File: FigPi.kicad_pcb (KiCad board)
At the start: 2 copper layers, 25.8 x 40.4 mm, 45 parts, among them J1 MOLEX_47346-100147346, J2 SPI0 / PWM2 / PWM3, J3 UART0 / PWM3 / PWM4, J4 STEMMA_1/QWIIC_1/I2C1/PMW1, J5 ADC / PWM5 / PWM6, J6 STEMMA_0/QWIIC_0/I2C0/PMW0, J7 PWR, SW1 KMS233GLFG, SW2 KMS233GLFG, U1 RP2040, U2 QSPI NOR FLASH 2MiB 2x3mm USO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, U3 AP2112K-3.3, U4 OT201612MJBA4SL

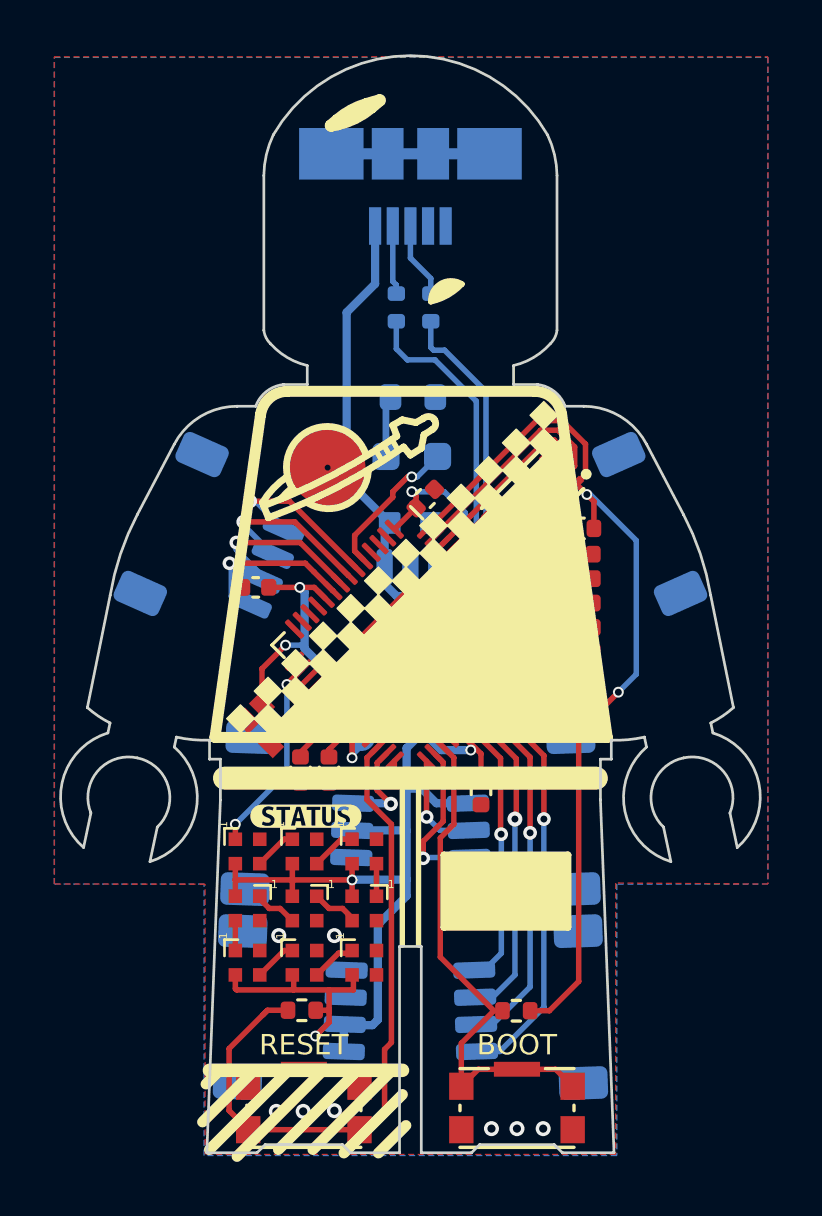
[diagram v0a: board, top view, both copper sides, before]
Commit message: Update to v2.3
Updated the schematic and board to v2.3.
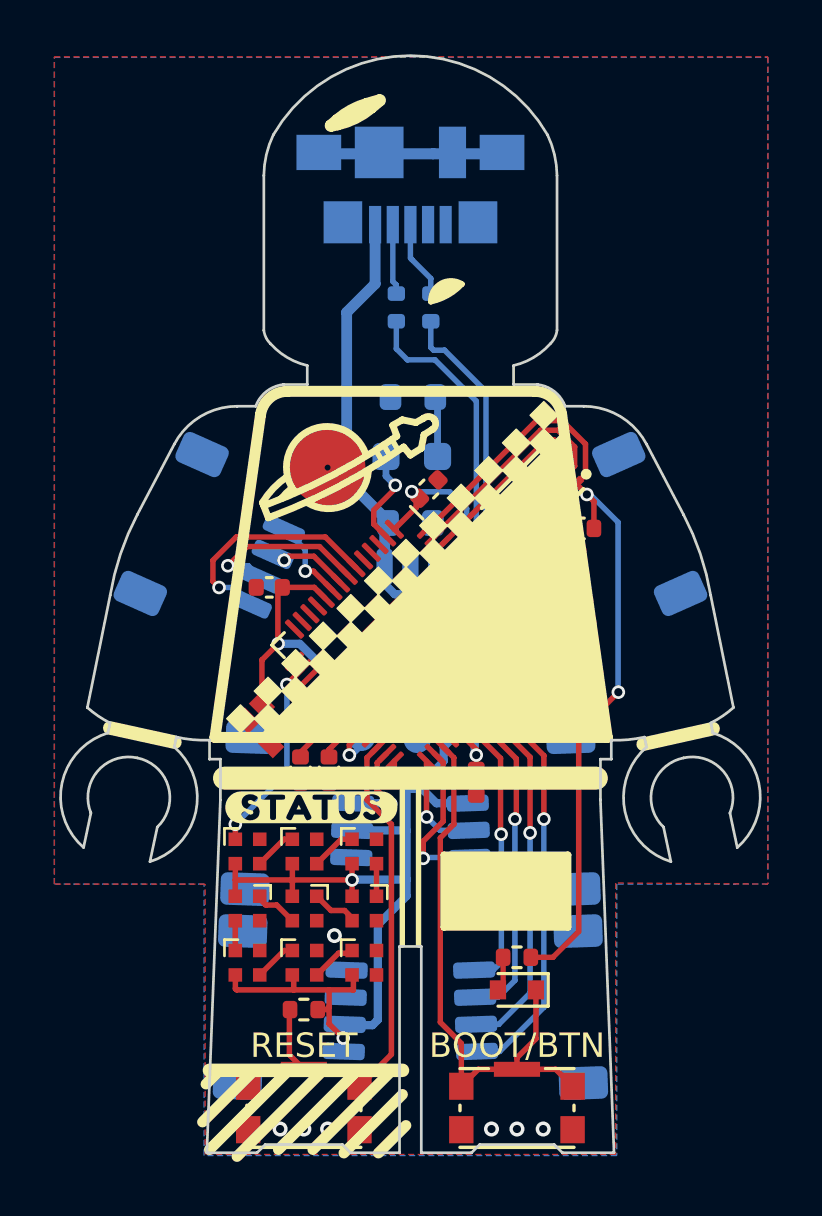
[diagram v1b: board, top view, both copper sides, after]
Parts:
- removed the J1 at (12.0, -36.8)
- removed kibuzzard-620D4CA4: G***, kibuzzard-620D4CA4
- added D11: RB520S-30, Diode_SMD:D_SOD-523, F.Cu at (15.9, -6.00)
- added J7: USB_B_Micro, Connector_USB:USB_Micro-B_Molex_47346-0001, B.Cu at (12.0, -35.6)
- added kibuzzard-640B746F: G***, kibuzzard-640B746F, F.Cu at (8.35, -12.7)
- added kibuzzard-640F7A39: G***, kibuzzard-640F7A39, B.Cu at (16.1, -16.5)
- added kibuzzard-640F7A5B: G***, kibuzzard-640F7A5B, B.Cu at (8.12, -16.5)
- added kibuzzard-640F7BF6: G***, kibuzzard-640F7BF6, B.Cu at (17.4, -26.2)
- added kibuzzard-640F7C1A: G***, kibuzzard-640F7C1A, B.Cu at (6.47, -26.4)
- added kibuzzard-640F7C6F: G***, kibuzzard-640F7C6F, B.Cu at (7.67, -1.18)
- added kibuzzard-640F7C7F: G***, kibuzzard-640F7C7F, B.Cu at (16.8, -1.15)
- added kibuzzard-640F7D7C: G***, kibuzzard-640F7D7C, B.Cu at (9.18, -32.5)
- C4: renamed from C9; footprint MINI_SAM_D51_r025_b001:0603_CAPACITOR -> Resistor_SMD:R_0603_1608Metric
- C5: renamed from C10; footprint MINI_SAM_D51_r025_b001:0603_CAPACITOR -> Resistor_SMD:R_0603_1608Metric
- SW1, SW2: value KMS233GLFG -> KMS231GLFG
- U2: value QSPI NOR FLASH 2MiB 2x3mm USON (W25Q16JVUXIQ) -> QSPI NOR FLASH 2MiB 2x3mm USON (W25Q16JVUXxQ)
- moved TP2 2.47 mm to (12.2, -15.2)
- moved R6 1.97 mm to (15.9, -7.20)
- moved C1 0.52 mm to (17.7, -22.1)
- moved C8 0.50 mm to (6.80, -20.8)
- moved C6 0.40 mm to (17.9, -21.1)
- moved C11 0.39 mm to (14.4, -13.7)
- moved C10 0.37 mm to (12.7, -24.4)
- moved C2 0.27 mm to (18.0, -20.2)
- moved C7 0.15 mm to (18.1, -19.4)
- moved C13 0.10 mm to (18.4, -17.6)
- moved R2 0.08 mm to (8.07, -5.28), turned to 0 degrees
- turned D10 to 180 degrees
- turned R1 to 180 degrees
- renumbered C11 to C10, C12 to C11, C13 to C12, C14 to C13, C5 to C6, C6 to C7, C7 to C8, C8 to C9, D2 to D1, D1 to D10, D5 to D2, D8 to D3, D3 to D4, D6 to D5, D9 to D6, D4 to D7, D7 to D8, D10 to D9, J7 to J1, J6 to J3, J3 to J5, J5 to J6, R7 to R1, R5 to R2, R4 to R3, R2 to R4, R1 to R5, R3 to R6, U4 to U3, U3 to U4
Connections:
- net /QSPI_CS renamed QSPI_CS
- net /QSPI_DATA[0] renamed QSPI_SD0
- net /QSPI_DATA[1] renamed QSPI_SD1
- net /QSPI_DATA[2] renamed QSPI_SD2
- net /QSPI_DATA[3] renamed QSPI_SD3
- net /QSPI_SCK renamed QSPI_SCK
- net /USBD+ renamed USBD+
- net /USBD- renamed USBD-
- net /VBUS renamed VBUS
- C10 pad 2: +3V3 -> +3.3V
- C11 pad 2: +3V3 -> +3.3V
- C12 pad 2: +3V3 -> +3.3V
- C13 pad 2: +3V3 -> +3.3V
- C5 pad 1: +3V3 -> +3.3V
- C6 pad 2: +3V3 -> +3.3V
- C7 pad 2: +3V3 -> +3.3V
- C8 pad 2: +3V3 -> +3.3V
- C9 pad 2: +3V3 -> +3.3V
- D1 pad 2: +3V3 -> +3.3V
- D10 pad 2: /LED_G -> LED
- D2 pad 2: +3V3 -> +3.3V
- D3 pad 2: +3V3 -> +3.3V
- D4 pad 2: +3V3 -> +3.3V
- D5 pad 2: +3V3 -> +3.3V
- D6 pad 2: +3V3 -> +3.3V
- D7 pad 2: +3V3 -> +3.3V
- D8 pad 2: +3V3 -> +3.3V
- D9 pad 2: +3V3 -> +3.3V
- J1 pad 1: +3V3 -> +3.3V
- J1 pad 2: +3V3 -> +3.3V
- J2 pad 1: /MOSI/D10 -> /MISO/D9
- J2 pad 2: /SCK/D8 -> /D14
- J2 pad 3: /D14 -> /SCK/D8
- J2 pad 4: /MISO/D9 -> /MOSI/D10
- J3 pad 2: +3V3 -> +3.3V
- J4 pad 2: +3V3 -> +3.3V
- R2 pad 1: +3V3 -> ~{RESET}
- R2 pad 2: /RUN -> +3.3V
- R3 pad 1: +3V3 -> +3.3V
- R6 pad 1: /~{USB_BOOT} -> Net-(D11-Pad2)
- SW1 pad 1: /RUN -> GND
- SW1 pad 2: GND -> ~{RESET}
- SW1 pad 3: GND -> ~{RESET}
- SW1 pad 4: GND -> ~{RESET}
- SW1 pad 5: /RUN -> GND
- SW2 pad 2: /~{USB_BOOT} -> BUTTON
- SW2 pad 3: /~{USB_BOOT} -> BUTTON
- SW2 pad 4: /~{USB_BOOT} -> BUTTON
- U1 pad 1: +3V3 -> +3.3V
- U1 pad 10: +3V3 -> +3.3V
- U1 pad 2: unconnected-(U1-Pad2) -> LED
- U1 pad 22: +3V3 -> +3.3V
- U1 pad 26: /RUN -> ~{RESET}
- U1 pad 31: /~{USB_BOOT} -> BUTTON
- U1 pad 33: +3V3 -> +3.3V
- U1 pad 42: +3V3 -> +3.3V
- U1 pad 43: +3V3 -> +3.3V
- U1 pad 44: +3V3 -> +3.3V
- U1 pad 48: +3V3 -> +3.3V
- U1 pad 49: +3V3 -> +3.3V
- U1 pad 5: /LED_G -> unconnected-(U1-Pad5)
- U2 pad 8: +3V3 -> +3.3V
- U3 pad 4: +3V3 -> +3.3V
- U4 pad 5: +3V3 -> +3.3V
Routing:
- net +3V3: track 102.0 -> 0.00 mm, vias 10 -> 0
- net +3.3V: track 0.00 -> 98.4 mm, vias 0 -> 9
- net /RUN: track 25.8 -> 0.00 mm
- net BUTTON: track 0.00 -> 21.1 mm
- net ~{RESET}: track 0.00 -> 20.6 mm
- net /~{USB_BOOT}: track 19.0 -> 0.00 mm
- net /LED_G: track 5.42 -> 0.00 mm, vias 1 -> 0
- net /SCK/D8: track 6.19 -> 2.55 mm
- net LED: track 0.00 -> 3.63 mm, vias 0 -> 1
- net /MOSI/D10: track 6.31 -> 3.21 mm
- net QSPI_CS: track 32.9 -> 30.8 mm
- net /MISO/D9: track 6.59 -> 8.60 mm
- net Net-(D11-Pad2): track 0.00 -> 1.28 mm
- net +1V2: track 18.4 -> 17.3 mm
- net GND: track 5.85 -> 6.23 mm, vias 13 -> 12
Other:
- rule pad_to_mask_clearance: 0.0508 -> 0
- board text added: "+"
- board text added: "-"
- board text added: "BOOT/BTN"
- board text added: "Fig Pi v2.3"
- board text removed: "BOOT"
- board text removed: "Fig Pi v2.2"
